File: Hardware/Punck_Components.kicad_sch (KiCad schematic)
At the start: 115 parts, among them J1 Conn_01x12_Female, J2 Conn_01x12_Female, J3 Conn_01x12_Female, J4 Conn_01x12_Female, J5 Debug_Header, J6 SWD_Header, J7 Eurorack_10_pin_power, Q1 MMBT3904, Q2 MMBT3904, Q3 MMBT3904, Q4 MMBT3904, Q5 MMBT3904, Q6 MMBT3904, Q7 MMBT3904, U1 TL074, U2 STM32H743ZITx, U3 W25Q128JVS, U4 PCM5100APW, U5 W25Q128JVS, U6 TPS561201, U7 LD1117-3.3-4Tab, Y1 8MHz 20pF

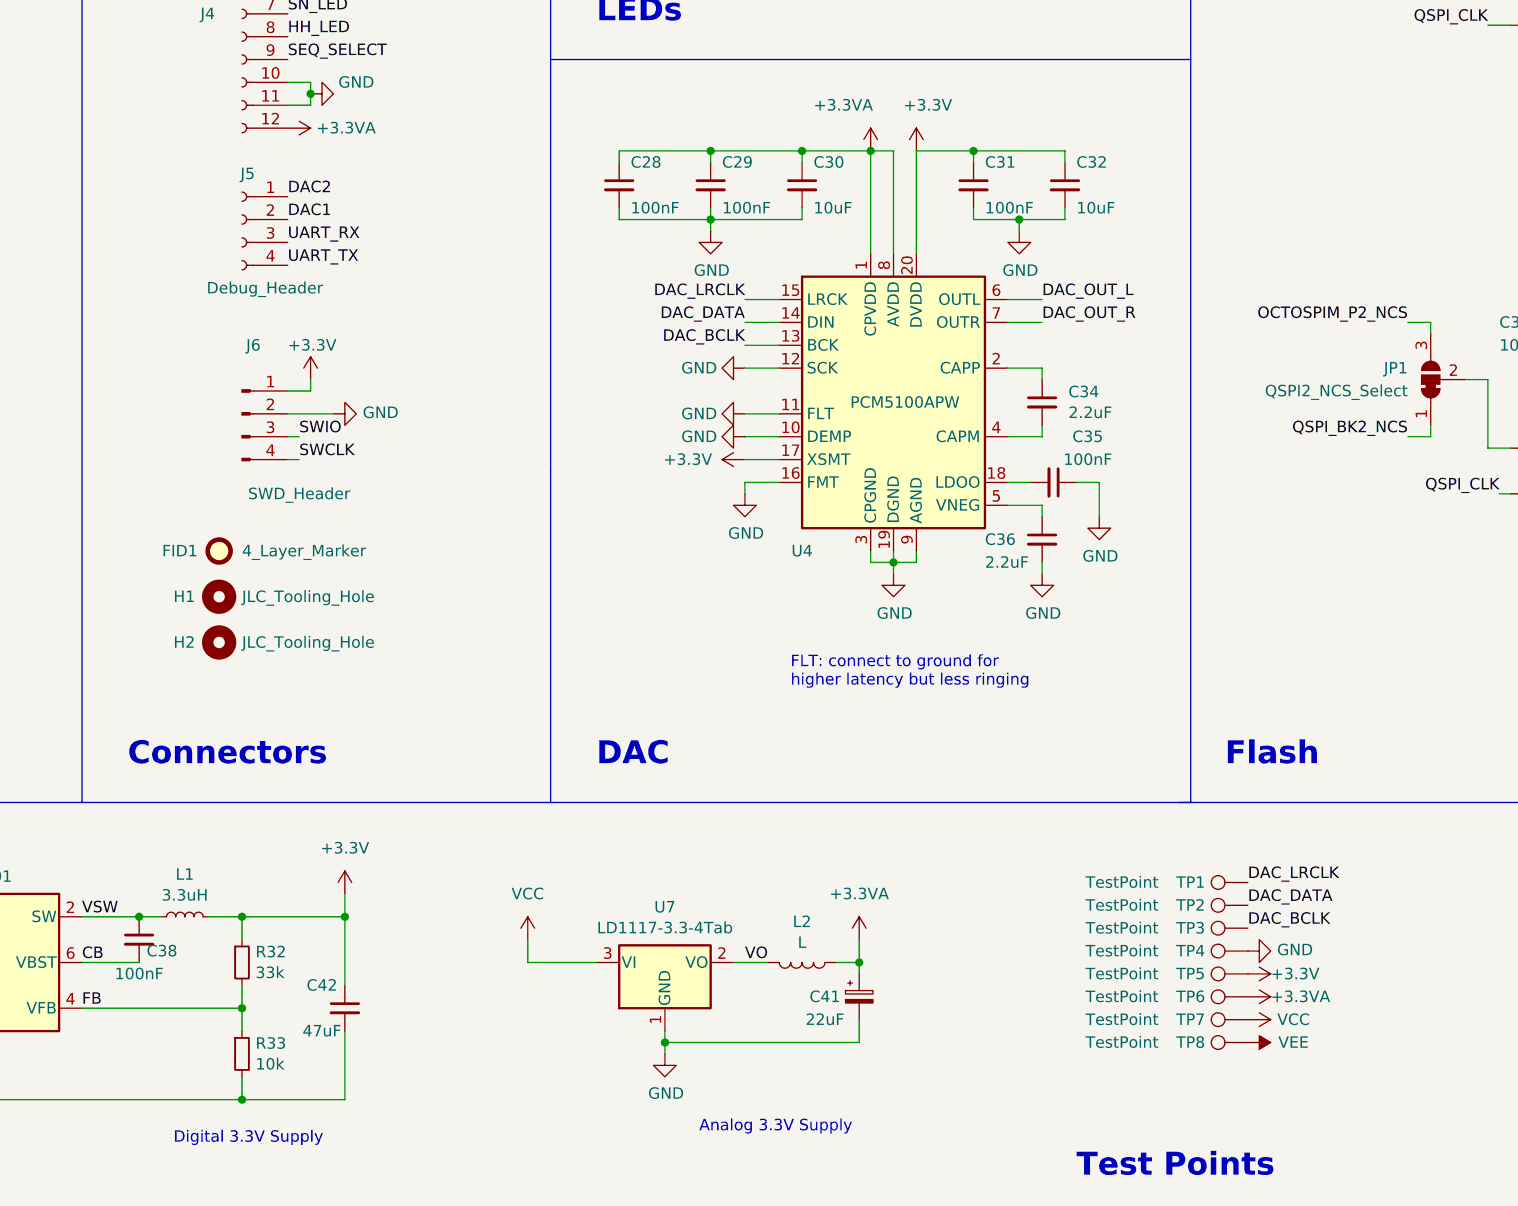
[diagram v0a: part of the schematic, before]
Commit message: Final tweaking and v1 gerber creation; JLC order placed
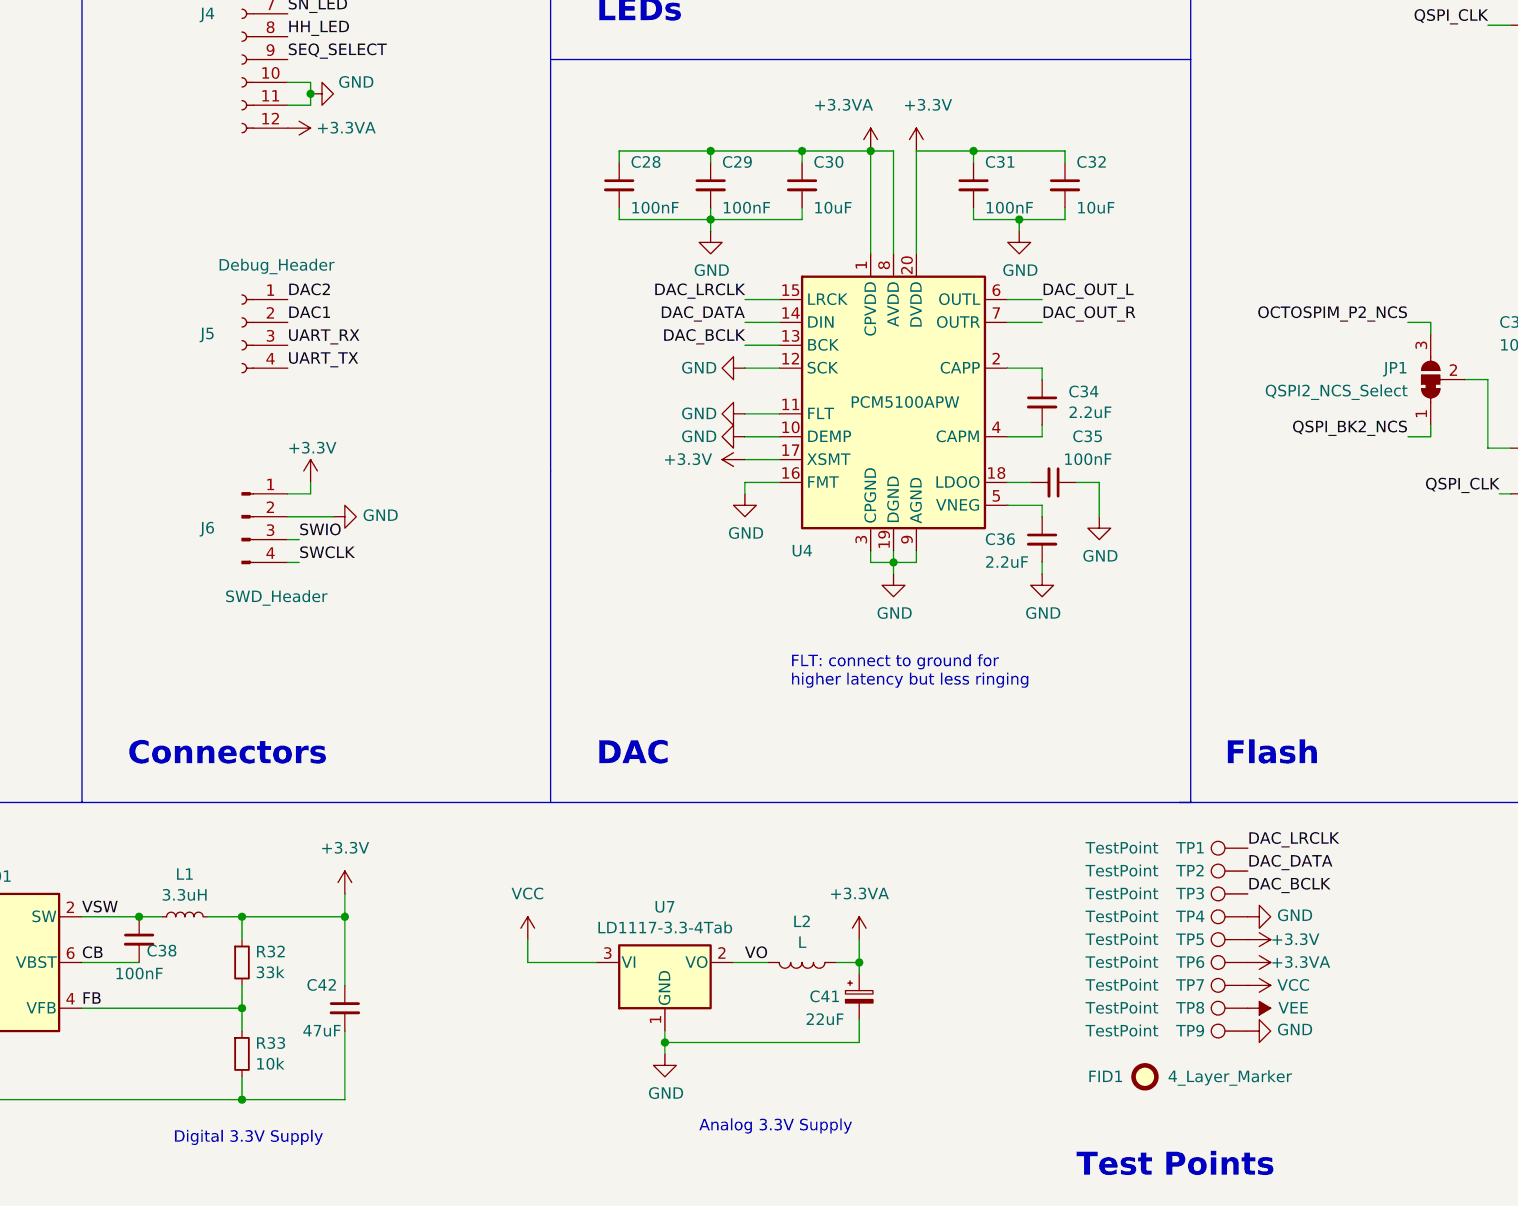
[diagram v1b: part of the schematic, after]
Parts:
- removed H1, H2: JLC_Tooling_Hole, Custom_Footprints:JLC_SMT_Tooling_Hole, symbol Mechanical:MountingHole
- added TP9: TestPoint, Custom_Footprints:1.3mm_Test_Point, symbol Connector:TestPoint
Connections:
- net GND: now also TP9.1
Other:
- moved on the sheet: FID1, J5, J6, TP1, TP2, TP3, TP4, TP5, TP6, TP7, TP8
